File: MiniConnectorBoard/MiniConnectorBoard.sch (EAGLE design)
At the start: 4 parts

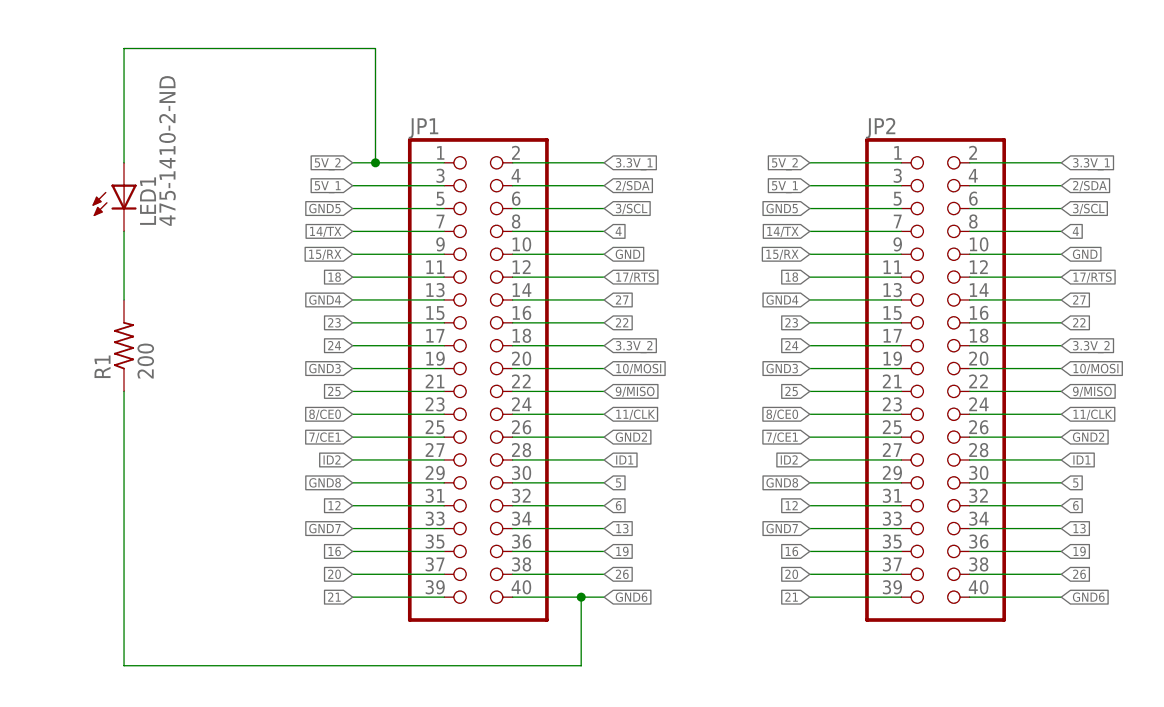
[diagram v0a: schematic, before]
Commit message: MiniConnectorBoard - first cut
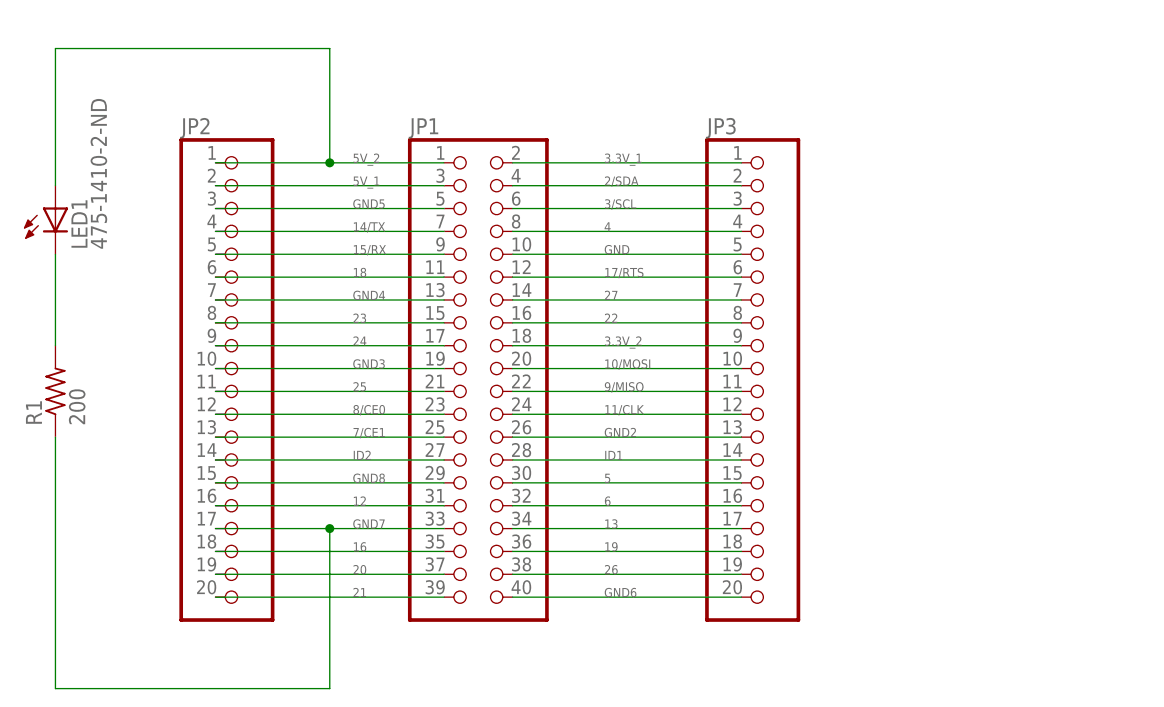
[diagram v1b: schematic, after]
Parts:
- added JP3: NONE, MiniConnectorBoard:PINHD-1X20
- JP2: device HeaderConnectorBoard:PINHD-2X20 -> MiniConnectorBoard:PINHD-1X20
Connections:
- net 10/MOSI: now also JP3.10; no longer JP2.20
- net 11/CLK: now also JP3.12; no longer JP2.24
- net 12: now also JP2.16; no longer JP2.31
- net 13: now also JP3.17; no longer JP2.34
- net 14/TX: now also JP2.4; no longer JP2.7
- net 15/RX: now also JP2.5; no longer JP2.9
- net 16: now also JP2.18; no longer JP2.35
- net 17/RTS: now also JP3.6; no longer JP2.12
- net 18: now also JP2.6; no longer JP2.11
- net 19: now also JP3.18; no longer JP2.36
- net 2/SDA: now also JP3.2; no longer JP2.4
- net 20: now also JP2.19; no longer JP2.37
- net 21: now also JP2.20; no longer JP2.39
- net 22: now also JP3.8; no longer JP2.16
- net 23: now also JP2.8; no longer JP2.15
- net 24: now also JP2.9; no longer JP2.17
- net 25: now also JP2.11; no longer JP2.21
- net 26: now also JP3.19; no longer JP2.38
- net 27: now also JP3.7; no longer JP2.14
- net 3.3V_1: now also JP3.1; no longer JP2.2
- net 3.3V_2: now also JP3.9; no longer JP2.18
- net 3/SCL: now also JP3.3; no longer JP2.6
- net 4: now also JP3.4; no longer JP2.8
- net 5: now also JP3.15; no longer JP2.30
- net 5V_1: now also JP2.2; no longer JP2.3
- net 6: now also JP3.16; no longer JP2.32
- net 7/CE1: now also JP2.13; no longer JP2.25
- net 8/CE0: now also JP2.12; no longer JP2.23
- net 9/MISO: now also JP3.11; no longer JP2.22
- net GND: now also JP3.5; no longer JP2.10
- net GND2: now also JP3.13; no longer JP2.26
- net GND3: now also JP2.10; no longer JP2.19
- net GND4: now also JP2.7; no longer JP2.13
- net GND5: now also JP2.3; no longer JP2.5
- net GND6: now also JP3.20; no longer JP2.40, R1.1
- net GND7: now also JP2.17, R1.1; no longer JP2.33
- net GND8: now also JP2.15; no longer JP2.29
- net ID1: now also JP3.14; no longer JP2.28
- net ID2: now also JP2.14; no longer JP2.27
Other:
- moved on the sheet: LED1, R1
